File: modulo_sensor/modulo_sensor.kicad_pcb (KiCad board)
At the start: 2 copper layers, 112.4 x 36.6 mm, 33 parts, among them J1 Conn_01x08_Pin, U1 74HC14DR2G

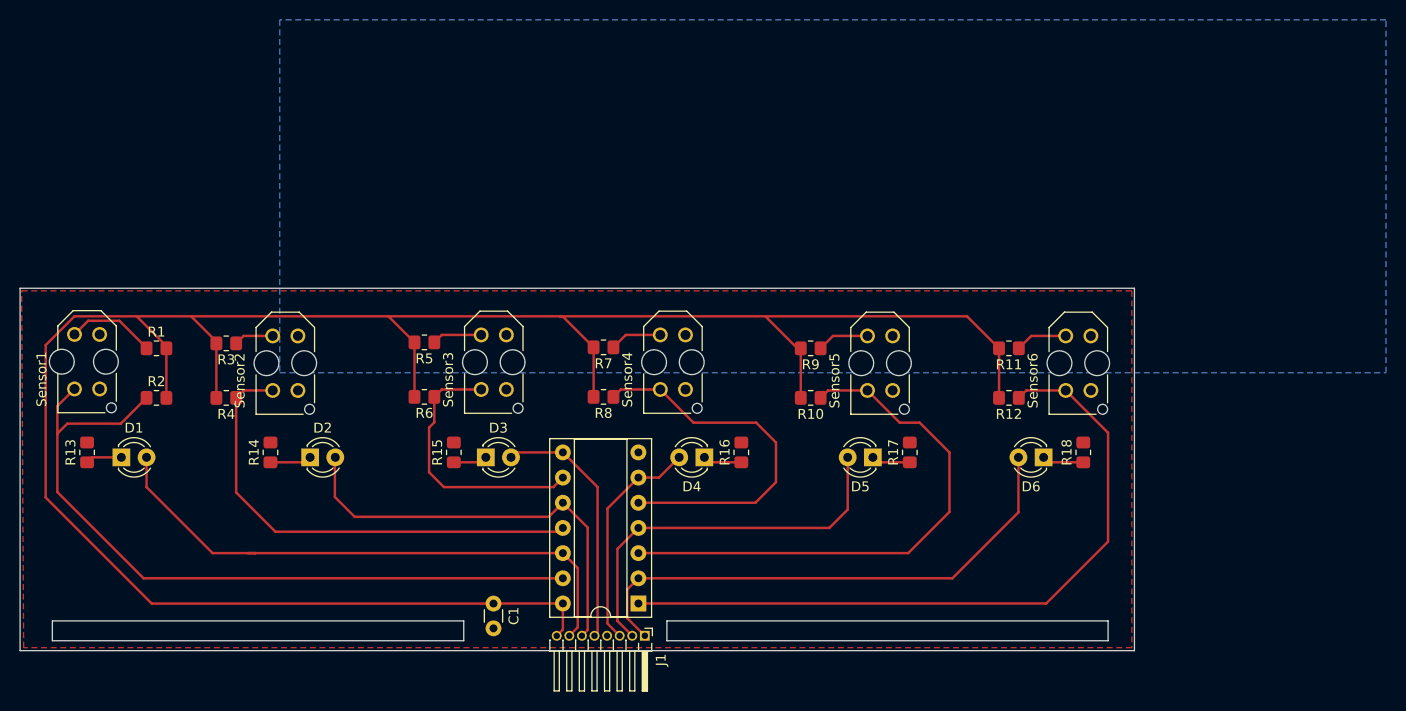
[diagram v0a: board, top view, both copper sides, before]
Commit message: fix: Guardo el archivo (fallo del commit anterior)
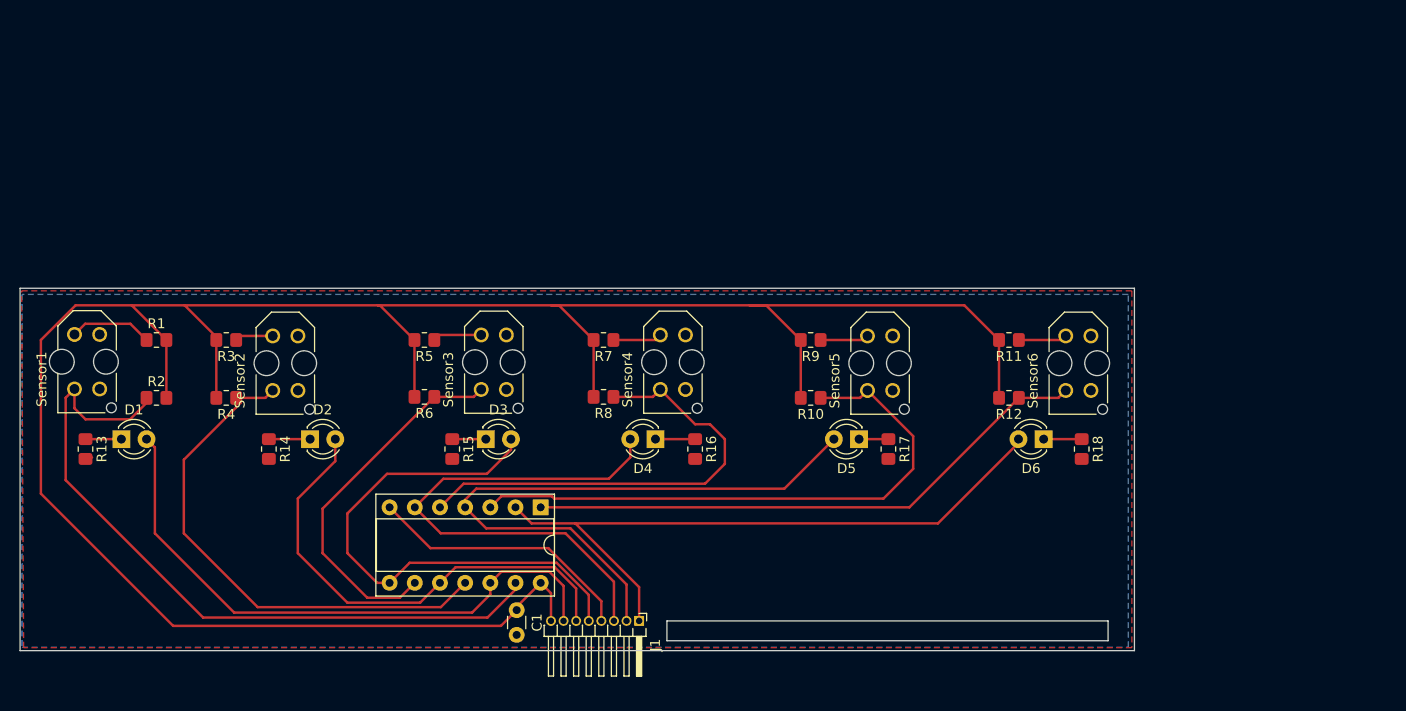
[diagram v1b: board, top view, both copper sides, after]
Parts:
- moved U1 13.8 mm to (94.9, 77.4), turned to -90 degrees
- moved D4 5.27 mm to (106.5, 70.5)
- moved R16 4.67 mm to (110.5, 71.5), turned to -90 degrees
- moved C1 2.43 mm to (92.5, 87.8)
- moved D5 2.31 mm to (127.0, 70.5)
- moved R17 2.19 mm to (130.0, 71.5), turned to -90 degrees
- moved D1 1.84 mm to (52.6, 70.5)
- moved D2 1.84 mm to (71.7, 70.5)
- moved D3 1.84 mm to (89.4, 70.5)
- moved D6 1.84 mm to (145.7, 70.5)
- moved J1 1.61 mm to (104.8, 88.8)
- moved R1 0.84 mm to (56.2, 60.5)
- moved R11 0.84 mm to (142.2, 60.5)
- moved R9 0.84 mm to (122.2, 60.5)
- moved R7 0.74 mm to (101.3, 60.5)
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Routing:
- net /Led_Sensor4: track 22.7 -> 52.8 mm
- net /Led_Sensor3: track 25.5 -> 54.6 mm
- net GND: track 0.62 -> 28.0 mm
- net /Led_Sensor5: track 39.5 -> 63.7 mm
- net /Sensor6: track 72.1 -> 57.9 mm
- net /Led_Sensor6: track 53.6 -> 67.7 mm
- net vcc: track 227.2 -> 239.4 mm
- net /Sensor3: track 27.4 -> 37.3 mm
- net /Sensor4: track 37.7 -> 46.7 mm
- net /Led_Sensor2: track 43.2 -> 48.9 mm
- net /Sensor5: track 55.0 -> 59.3 mm
- net /Sensor2: track 48.3 -> 52.3 mm
- net /Led_Sensor1: track 57.9 -> 60.9 mm
- net /Sensor1: track 76.2 -> 73.4 mm
- net Net-(D5-K): track 3.93 -> 2.96 mm
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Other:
- outline, holes or cut-outs redrawn
